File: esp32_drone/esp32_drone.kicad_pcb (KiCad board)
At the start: 2 copper layers, 34.7 x 36.5 mm, 38 parts, among them J1 EE_SOCKET_01x01, J11 EE_SOCKET_01x07, J12 EE_SOCKET_01x07, J2 EE_SOCKET_01x01, J3 EE_SOCKET_01x01, J4 EE_SOCKET_01x01, J5 EE_SOCKET_01x01, J6 EE_SOCKET_01x01, J7 EE_SOCKET_01x01, J8 EE_SOCKET_01x01, J9 Conn_01x02_Pin, Q1 AO3400A, Q2 AO3400A, Q3 AO3400A, Q4 AO3400A, U1 AP2204K-ADJ, U2 MPU-6050

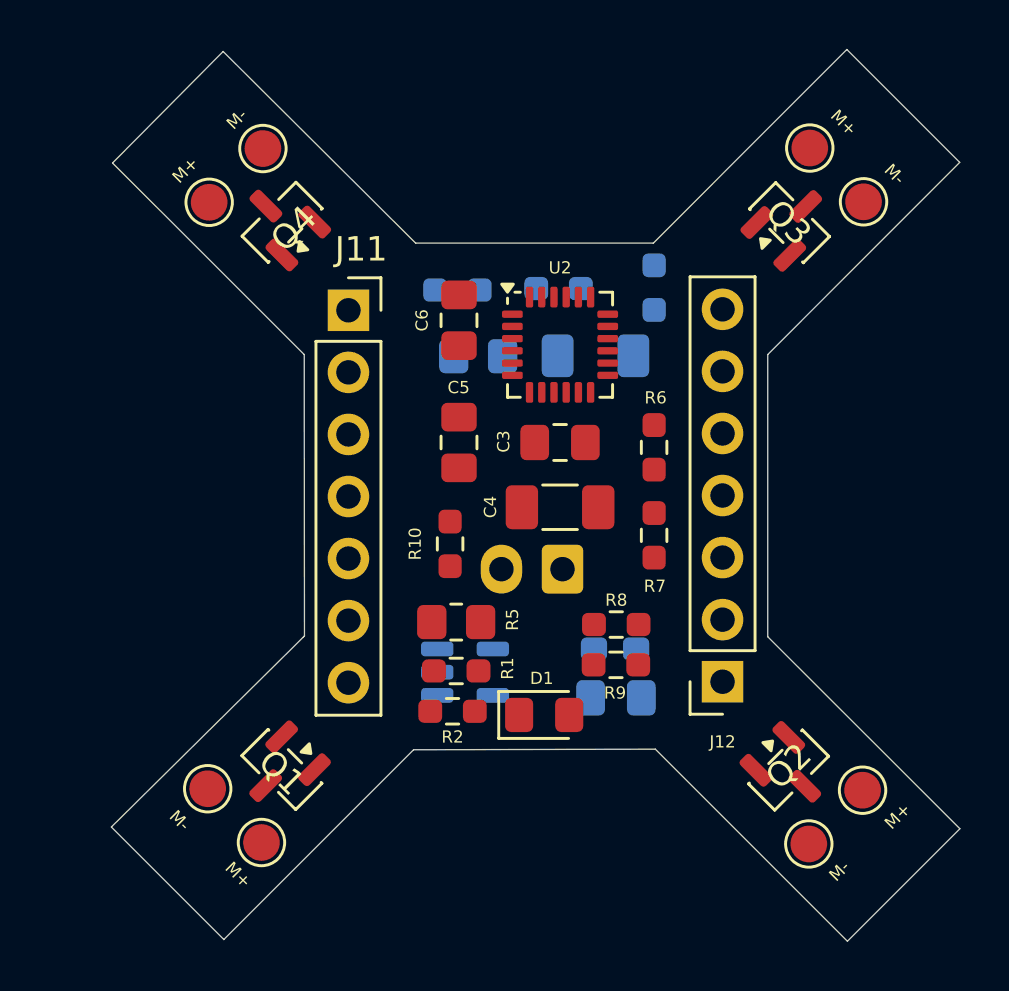
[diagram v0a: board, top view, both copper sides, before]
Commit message: finished routing
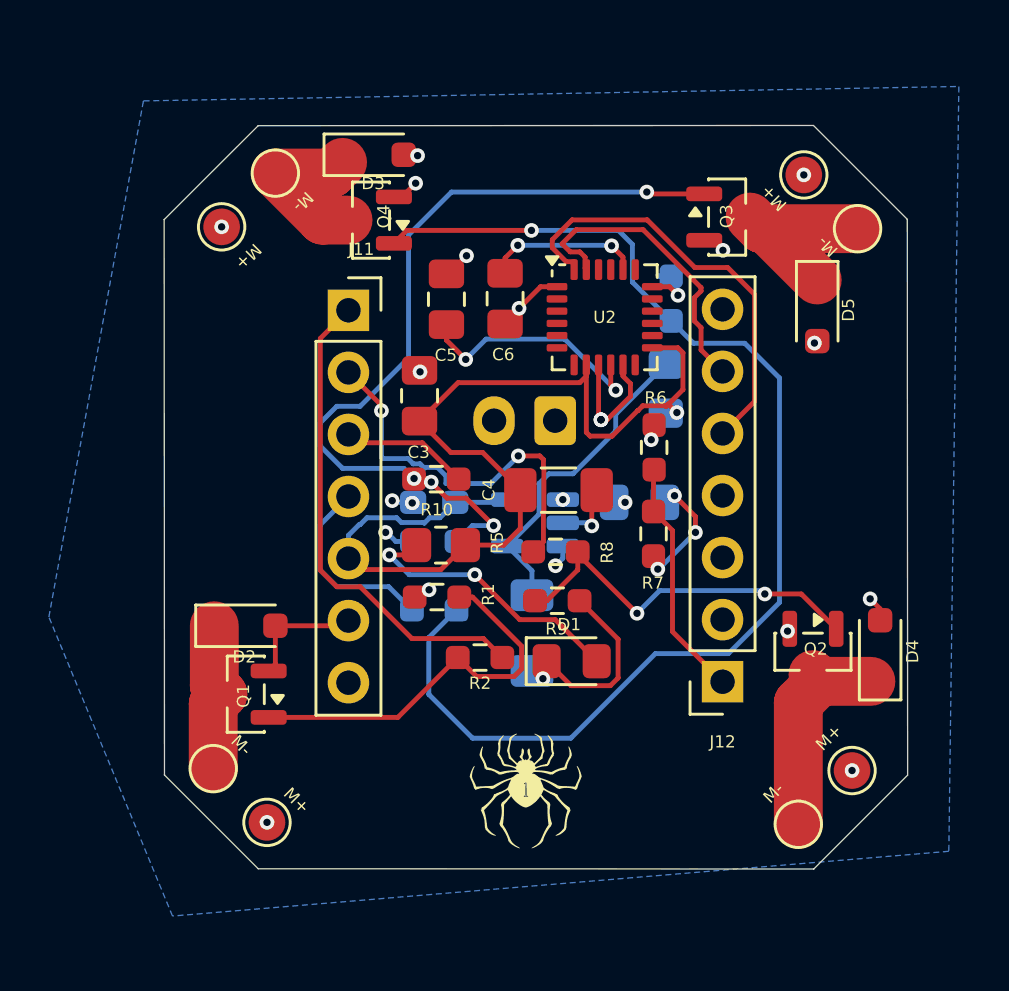
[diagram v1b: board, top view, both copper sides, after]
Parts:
- added D2: UF4007, Diode_SMD:D_SOD-323_HandSoldering, F.Cu at (111.2, 81.2)
- added D3: UF4007, Diode_SMD:D_SOD-323_HandSoldering, F.Cu at (116.5, 62.0)
- added D4: UF4007, Diode_SMD:D_SOD-323_HandSoldering, F.Cu at (137.2, 82.3)
- added D5: UF4007, Diode_SMD:D_SOD-323_HandSoldering, F.Cu at (134.7, 68.3)
- G***: moved to F.Cu
- moved R12 14.1 mm to (119.0, 80.6), turned to 0 degrees
- moved R11 13.7 mm to (119.0, 77.8), turned to 180 degrees
- moved R4 11.6 mm to (123.0, 81.5), turned to -90 degrees
- moved G*** 11.0 mm to (122.7, 88.0), turned to 0 degrees
- moved C2 9.53 mm to (119.0, 76.2), turned to 180 degrees
- moved R13 8.76 mm to (128.7, 67.9), turned to 90 degrees
- moved C1 8.06 mm to (127.4, 76.2)
- moved R3 7.79 mm to (128.5, 71.5), turned to 90 degrees
- moved U1 6.75 mm to (123.1, 77.0), turned to 180 degrees
- moved J9 6.08 mm to (124.0, 72.9)
- moved C3 6.06 mm to (118.4, 71.8), turned to 90 degrees
- moved C5 5.89 mm to (119.5, 67.9)
- moved Q2 4.94 mm to (134.5, 82.3), turned to -90 degrees
- moved R8 3.88 mm to (124.0, 78.2)
- moved Q4 3.64 mm to (116.4, 64.7), turned to 180 degrees
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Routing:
- net VCC: track 0.00 -> 86.4 mm, vias 0 -> 8
- net Net-(Q4-G): track 0.00 -> 50.4 mm, vias 0 -> 1
- net /3V3: track 0.00 -> 42.3 mm, vias 0 -> 1
- net GND: track 0.00 -> 40.3 mm, vias 0 -> 21
- net Net-(Q3-G): track 0.00 -> 33.8 mm, vias 0 -> 4
- net /PWM1: track 0.00 -> 20.0 mm
- net /SDA: track 0.00 -> 17.9 mm
- net Net-(Q1-G): track 0.00 -> 16.1 mm
- net /PWM2: track 0.00 -> 15.8 mm, vias 0 -> 2
- net Net-(Q2-G): track 0.00 -> 15.7 mm, vias 0 -> 2
- net Net-(U1-ADJ): track 0.00 -> 13.1 mm
- net /SCL: track 0.00 -> 12.6 mm
- net Net-(D1-A): track 0.00 -> 11.6 mm, vias 0 -> 2
- net Net-(U2-REGOUT): track 0.00 -> 10.2 mm, vias 0 -> 2
- net /A0: track 0.00 -> 9.86 mm
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- added copper zone on B.Cu, net GND
- added copper zone on In1.Cu, net GND
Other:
- board size 34.7 x 36.5 mm -> 30.4 x 30.4 mm
- copper layers 2 -> 4
